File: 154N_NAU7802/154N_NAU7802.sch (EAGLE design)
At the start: 25 parts, among them IC1 MCP604SL, J4 1725698, J5 1725698, U3 NAU7802, U4 LMV324

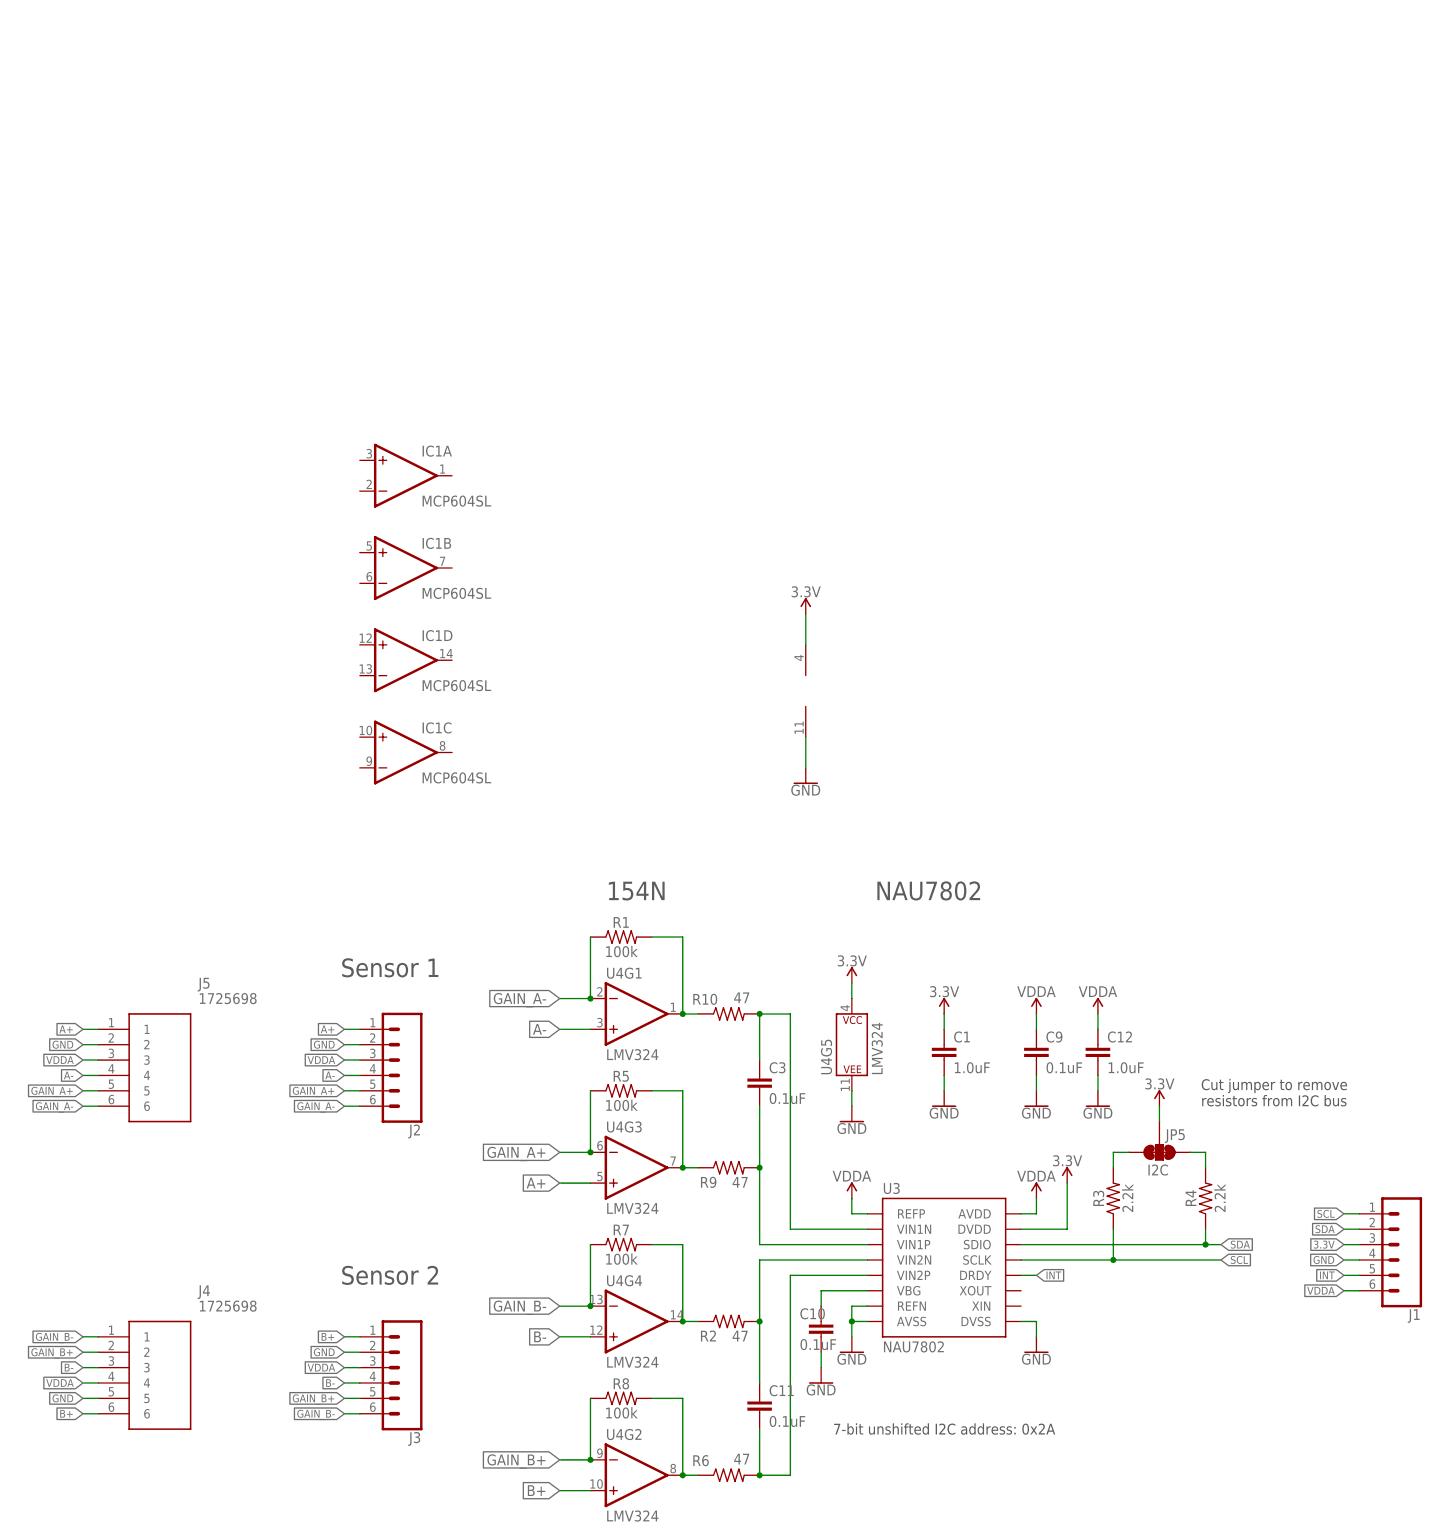
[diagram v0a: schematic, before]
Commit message: Lagopus 3.0 order
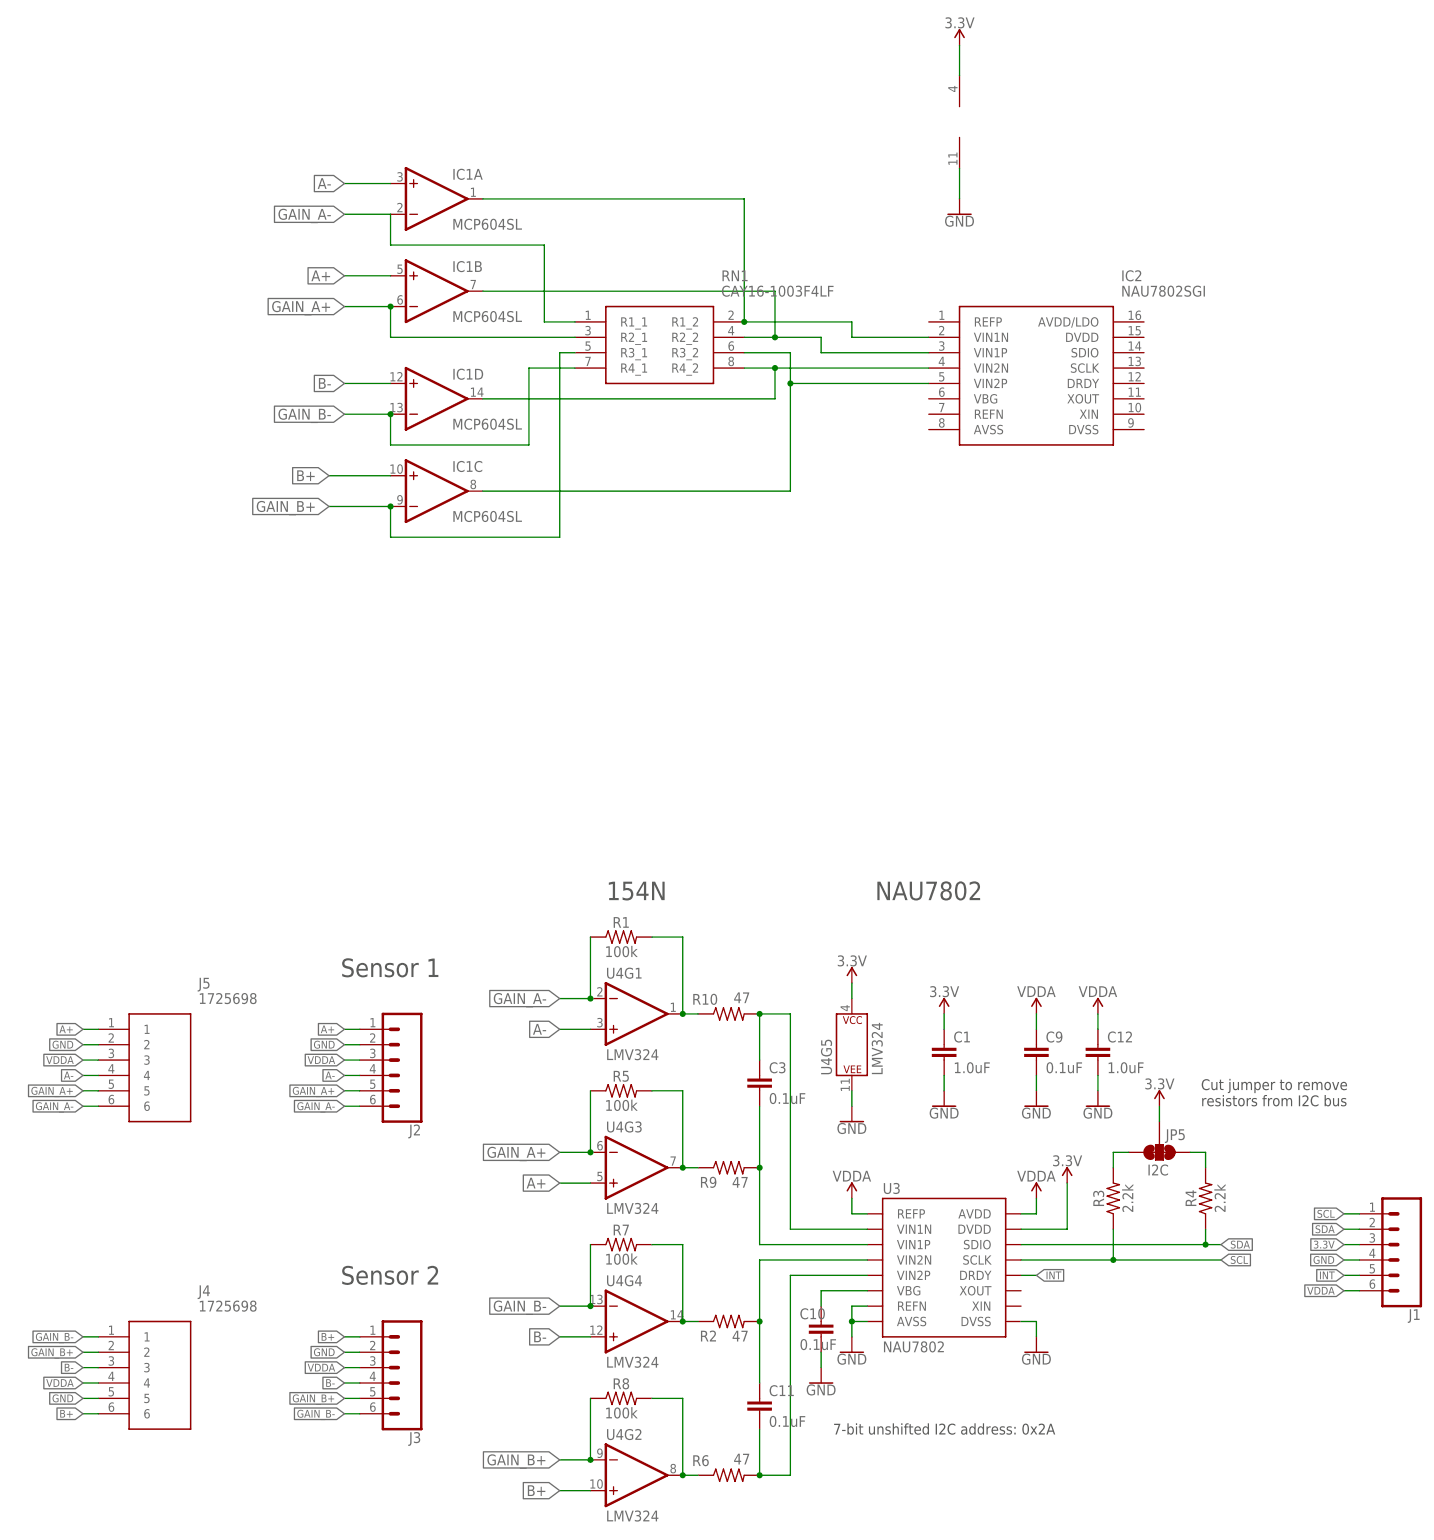
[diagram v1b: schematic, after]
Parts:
- added IC2: NAU7802SGI, NAU7802SGI:NAU7802SGI
- added RN1: CAY16-1003F4LF, CAY16-1003F4LF:CAY16-1003F4LF
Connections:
- new net N$16: IC1C.OUT, IC2.VIN2P, RN1.R3_2
- new net N$5: IC1A.OUT, IC2.VIN1N, RN1.R1_2
- new net N$7: IC1B.OUT, IC2.VIN1P, RN1.R2_2
- new net N$8: IC1D.OUT, IC2.VIN2N, RN1.R4_2
- net A+: now also IC1B.+IN
- net A-: now also IC1A.+IN
- net B+: now also IC1C.+IN
- net B-: now also IC1D.+IN
- net GAIN_A+: now also IC1B.-IN, RN1.R2_1
- net GAIN_A-: now also IC1A.-IN, RN1.R1_1
- net GAIN_B+: now also IC1C.-IN, RN1.R3_1
- net GAIN_B-: now also IC1D.-IN, RN1.R4_1
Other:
- moved on the sheet: IC1A, IC1B, IC1C, IC1D
